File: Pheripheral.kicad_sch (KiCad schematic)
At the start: 1 part

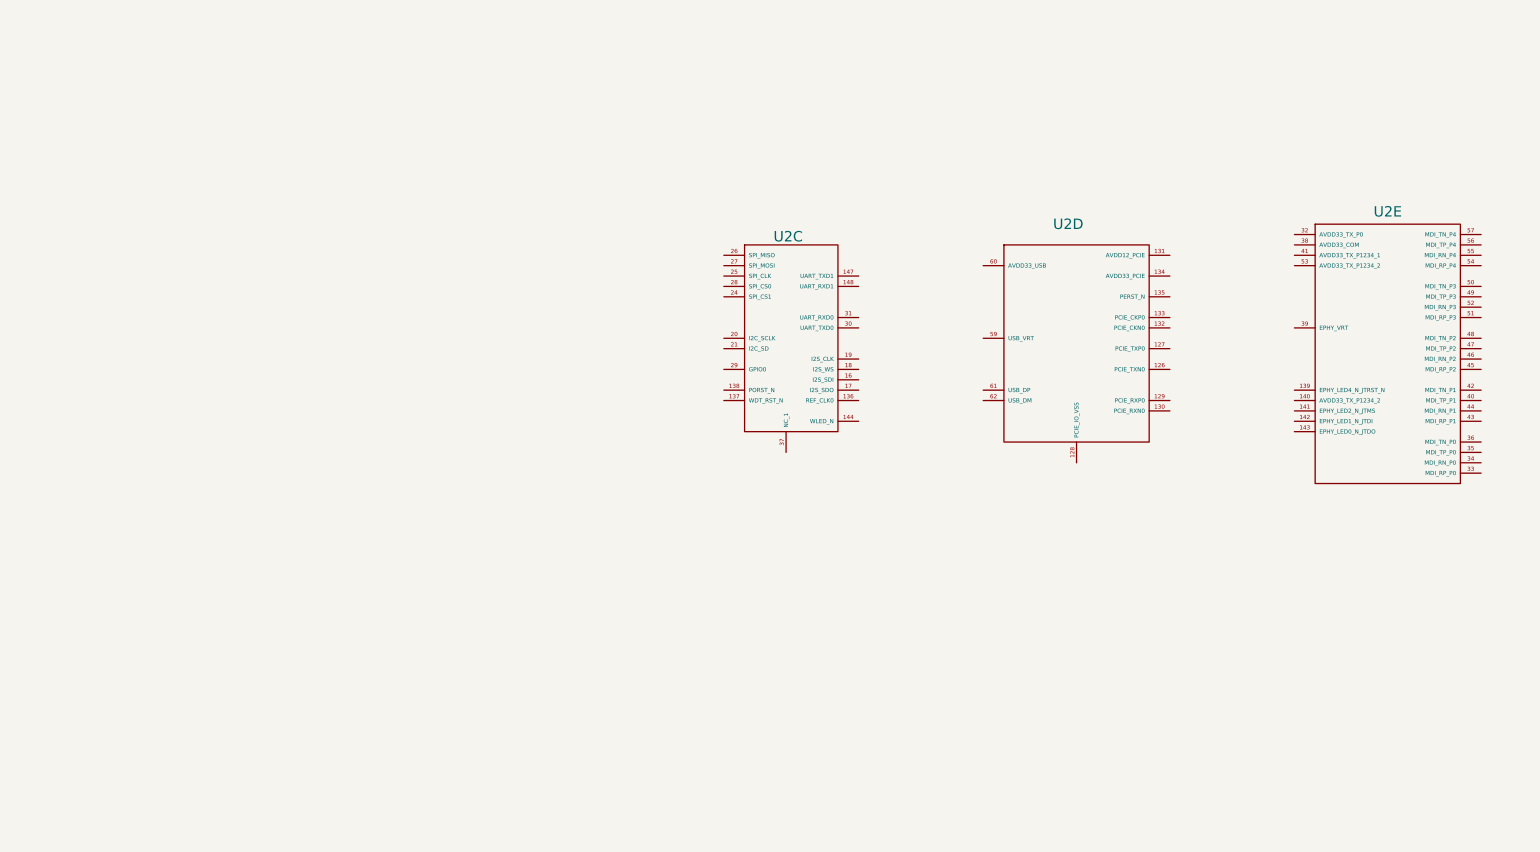
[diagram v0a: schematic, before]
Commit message: updated aux
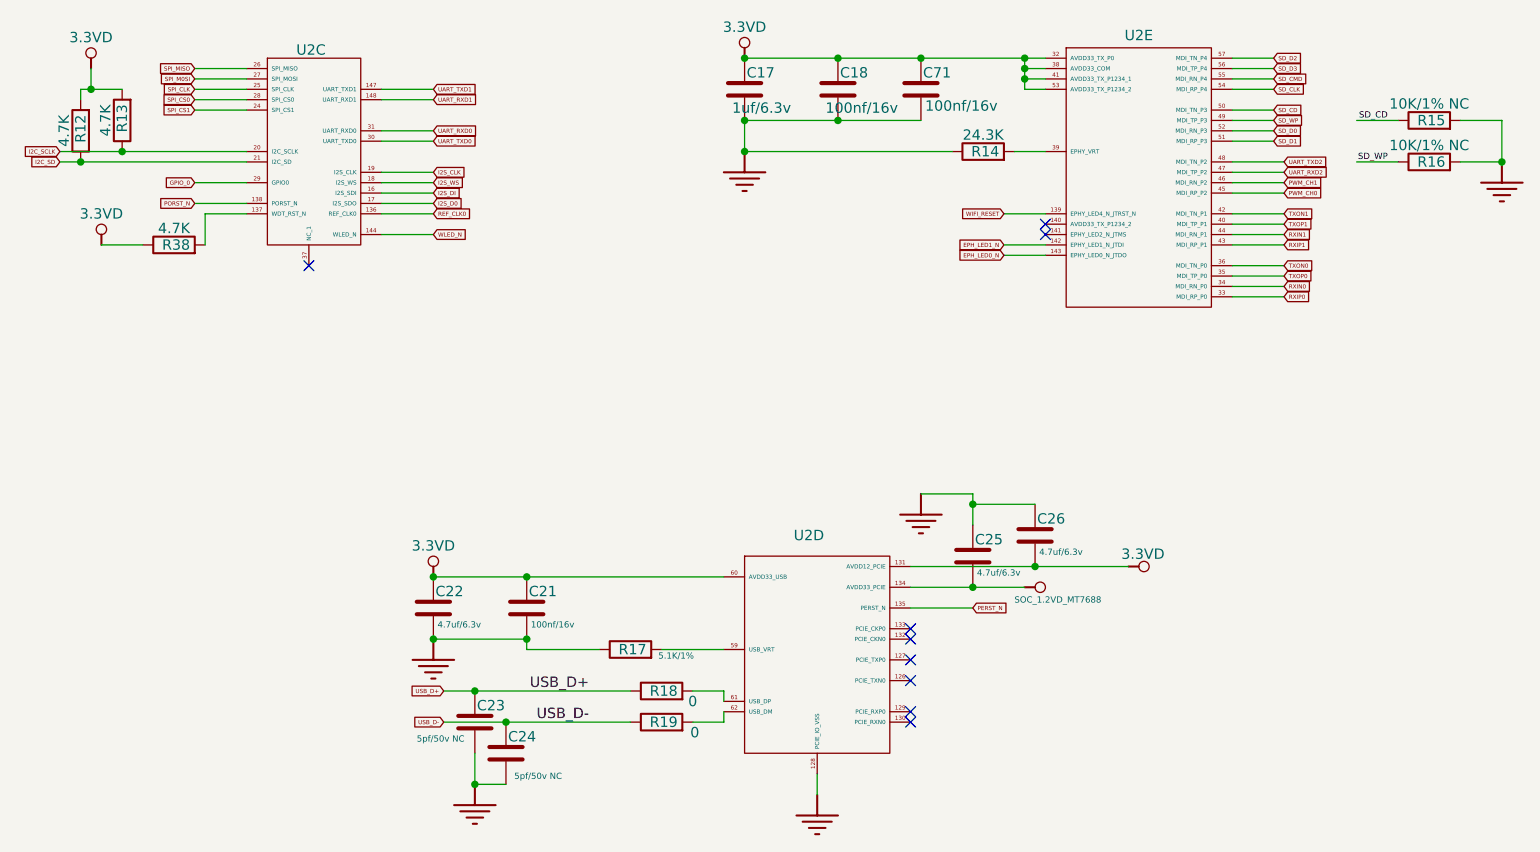
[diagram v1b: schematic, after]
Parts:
- added C17: 1uf/6.3v, symbol Device:C
- added C18, C21, C71: 100nf/16v, symbol Device:C
- added C22, C25, C26: 4.7uf/6.3v, symbol Device:C
- added C23, C24: 5pf/50v NC, symbol Device:C
- added R12, R13, R38: 4.7K, symbol Device:R
- added R14: 24.3K, symbol Device:R
- added R15, R16: 10K/1% NC, symbol Device:R
- added R17: 5.1K/1%, symbol Device:R
- added R18, R19: 0, symbol Device:R
- U2: footprint (none) -> MT7628:MT7628_footprint
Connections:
- net REF_CLK0: now reaches U2.136 (REF_CLK0)
- net at U2.137 (WDT_RST_N): now also R38.2
- net PORST_N: now reaches U2.138 (PORST_N)
- net WLED_N: now reaches U2.144 (WLED_N)
- net UART_TXD1: now reaches U2.147 (UART_TXD1)
- net UART_RXD1: now reaches U2.148 (UART_RXD1)
- net I2S_DI: now reaches U2.16 (I2S_SDI)
- net I2S_D0: now reaches U2.17 (I2S_SDO)
- net I2S_WS: now reaches U2.18 (I2S_WS)
- net I2S_CLK: now reaches U2.19 (I2S_CLK)
- net I2C_SCLK: now reaches U2.20 (I2C_SCLK)
- net I2C_SCLK: now also R13.1
- net I2C_SD: now reaches U2.21 (I2C_SD)
- net I2C_SD: now also R12.1
- net SPI_CS1: now reaches U2.24 (SPI_CS1)
- net SPI_CLK: now reaches U2.25 (SPI_CLK)
- net SPI_MISO: now reaches U2.26 (SPI_MISO)
- net SPI_M0SI: now reaches U2.27 (SPI_MOSI)
- net SPI_CS0: now reaches U2.28 (SPI_CS0)
- net GPIO_0: now reaches U2.29 (GPIO0)
- net UART_TXD0: now reaches U2.30 (UART_TXD0)
- net UART_RXD0: now reaches U2.31 (UART_RXD0)
- net WIFI_RESET: now reaches U2.139 (EPHY_LED4_N_JTRST_N)
- net EPH_LED1_N: now reaches U2.142 (EPHY_LED1_N_JTDI)
- net EPH_LED0_N: now reaches U2.143 (EPHY_LED0_N_JTDO)
- net 3.3VD: now reaches U2.32 (AVDD33_TX_P0)
- net 3.3VD: now also U2.131 (AVDD12_PCIE), U2.38 (AVDD33_COM), U2.41 (AVDD33_TX_P1234_1), U2.53 (AVDD33_TX_P1234_2), U2.60 (AVDD33_USB), C17.1, C18.1, C21.1, C22.1, C26.2, C71.1, R12.2, R13.2, R38.1
- net RXIP0: now reaches U2.33 (MDI_RP_P0)
- net RXIN0: now reaches U2.34 (MDI_RN_P0)
- net TXOP0: now reaches U2.35 (MDI_TP_P0)
- net TXON0: now reaches U2.36 (MDI_TN_P0)
- net at U2.39 (EPHY_VRT): now also R14.2
- net TXOP1: now reaches U2.40 (MDI_TP_P1)
- net TXON1: now reaches U2.42 (MDI_TN_P1)
- net RXIP1: now reaches U2.43 (MDI_RP_P1)
- net RXIN1: now reaches U2.44 (MDI_RN_P1)
- net PWM_CH0: now reaches U2.45 (MDI_RP_P2)
- net PWM_CH1: now reaches U2.46 (MDI_RN_P2)
- net UART_RXD2: now reaches U2.47 (MDI_TP_P2)
- net UART_TXD2: now reaches U2.48 (MDI_TN_P2)
- net SD_WP: now reaches U2.49 (MDI_TP_P3)
- net SD_WP: now also R16.1
- net SD_CD: now reaches U2.50 (MDI_TN_P3)
- net SD_CD: now also R15.1
- net SD_D1: now reaches U2.51 (MDI_RP_P3)
- net SD_D0: now reaches U2.52 (MDI_RN_P3)
- net SD_CLK: now reaches U2.54 (MDI_RP_P4)
- net SD_CMD: now reaches U2.55 (MDI_RN_P4)
- net SD_D3: now reaches U2.56 (MDI_TP_P4)
- net SD_D2: now reaches U2.57 (MDI_TN_P4)
- net GND: now reaches U2.128 (PCIE_IO_VSS)
- net GND: now also C17.2, C18.2, C21.2, C22.2, C23.2, C24.2, C25.1, C26.1, C71.2, R14.1, R15.2, R16.2, R17.1
- net SOC_1.2VD_MT7688: now reaches U2.134 (AVDD33_PCIE)
- net SOC_1.2VD_MT7688: now also C25.2
- net PERST_N: now reaches U2.135 (PERST_N)
- net at U2.59 (USB_VRT): now also R17.2
- net at U2.61 (USB_DP): now also R18.2
- net at U2.62 (USB_DM): now also R19.2
- new net USB_D+: C23.1, R18.1
- new net USB_D-: C24.1, R19.1
- no-connect marks 0 -> 9
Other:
- moved on the sheet: U2C, U2D, U2E

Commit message: init_sch
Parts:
- R12, R13, R38: footprint (none) -> Resistor_SMD:R_0402_1005Metric; LCSC (none) -> C25900
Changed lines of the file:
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@@
 			)
 		)
-		(property "Footprint" ""
+		(property "Footprint" "Resistor_SMD:R_0402_1005Metric"
 			(at 45.72 51.308 90)
 			(effects
@@
 		(property "Description" "Resistor"
 			(at 45.72 49.53 0)
+			(effects
+				(font
+					(size 1.27 1.27)
+				)
+				(hide yes)
+			)
+		)
+		(property "LCSC" "C25900"
+			(at 45.72 49.53 90)
 			(effects
 				(font
@@
 			)
 		)
-		(property "Footprint" ""
+		(property "Footprint" "Resistor_SMD:R_0402_1005Metric"
 			(at 36.068 35.56 90)
 			(effects
@@
 		(property "Description" "Resistor"
 			(at 34.29 35.56 0)
+			(effects
+				(font
+					(size 1.27 1.27)
+				)
+				(hide yes)
+			)
+		)
+		(property "LCSC" "C25900"
+			(at 34.29 35.56 90)
 			(effects
 				(font
@@
 			)
 		)
-		(property "Footprint" ""
+		(property "Footprint" "Resistor_SMD:R_0402_1005Metric"
 			(at 41.148 34.29 90)
 			(effects
@@
 			(effects
 				(font
+					(size 1.27 1.27)
+				)
+				(hide yes)
+			)
+		)
+		(property "LCSC" "C25900"
+			(at 39.37 34.29 90)
+			(effects
+				(font
